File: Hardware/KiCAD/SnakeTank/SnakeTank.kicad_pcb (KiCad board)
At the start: 4 copper layers, 80.5 x 36.6 mm, 51 parts, among them J1 Conn_01x12, J2 USB_C_Receptacle_USB2.0_16P, J3 RJ45, Q1 L8050QLT1G, Q2 L8050QLT1G, U1 LP2985-3.3, U2 ESP32-S3-WROOM-1-N8, U4 FT231XS

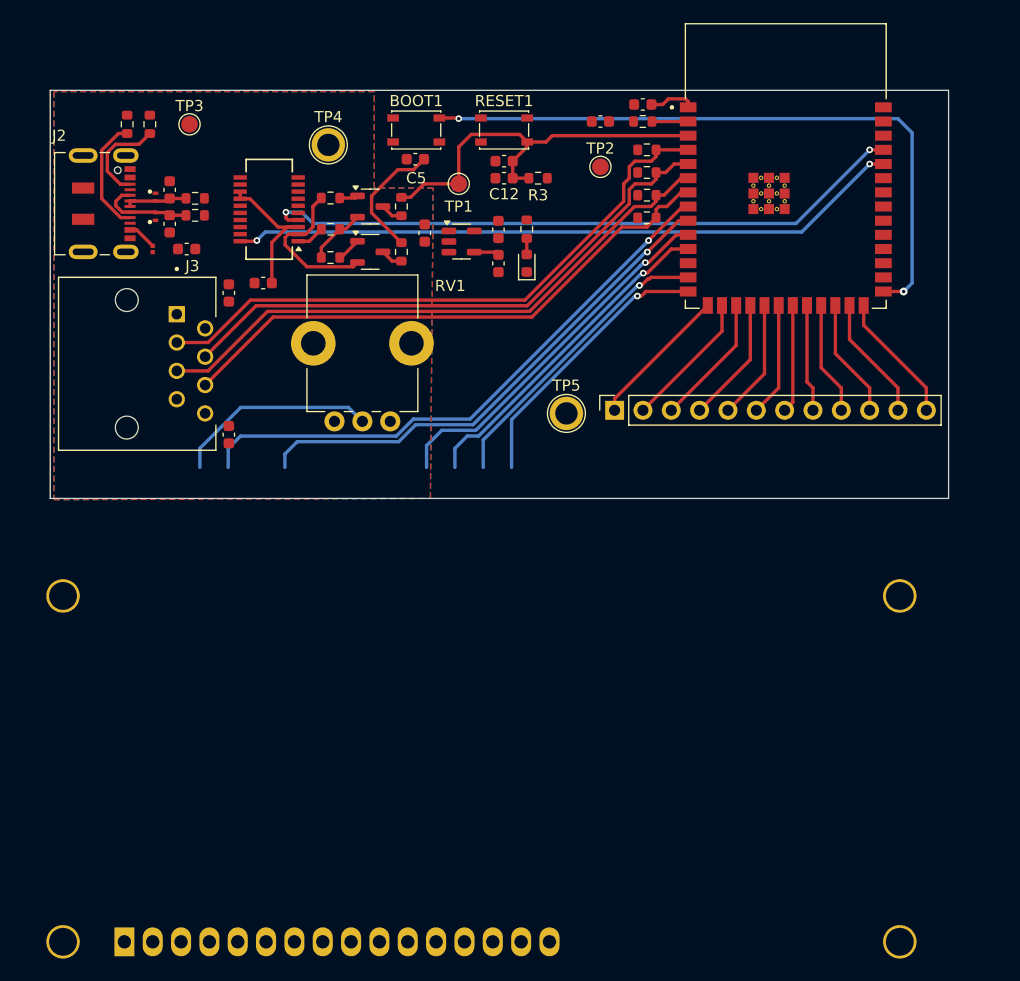
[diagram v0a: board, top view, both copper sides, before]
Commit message: WOOOHOO
rough draft of layout done
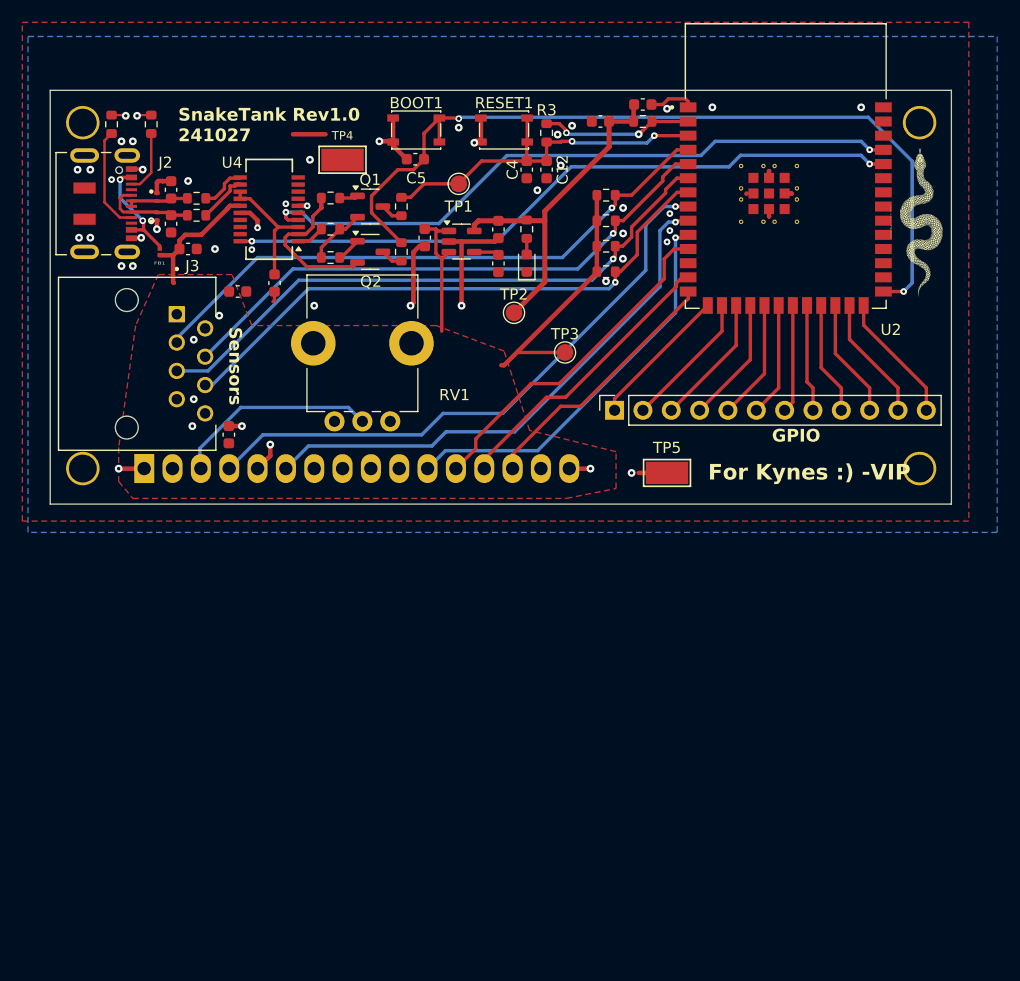
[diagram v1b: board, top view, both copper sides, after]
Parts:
- added G***: LOGO, graphics:snakeLogo, F.Cu at (95.9, 35.9)
- TP4, TP5: footprint TestPoint:TestPoint_Plated_Hole_D2.0mm -> TestPoint:TestPoint_Keystone_5019_Minature
- moved DS1 42.5 mm to (26.4, 58.0)
- moved TP3 39.4 mm to (64.1, 47.6)
- moved TP2 15.2 mm to (59.6, 44.1)
- moved TP5 10.5 mm to (73.3, 58.4)
- moved R12 6.05 mm to (67.8, 40.4)
- moved R13 5.85 mm to (67.8, 38.1)
- moved R14 5.66 mm to (67.8, 35.8)
- moved R15 5.47 mm to (67.8, 33.5)
- moved R3 4.13 mm to (62.5, 27.9), turned to -90 degrees
- moved C12 3.89 mm to (62.5, 31.2), turned to -90 degrees
- moved C4 2.17 mm to (60.7, 31.2), turned to -90 degrees
- moved TP4 1.84 mm to (44.2, 30.4)
- moved R1 1.40 mm to (23.5, 27.2)
- moved C7 1.02 mm to (38.1, 41.4), turned to -90 degrees
- moved C14 0.80 mm to (34.8, 42.2), turned to 0 degrees
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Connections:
- U2 pad 41_10: (no net) -> GND
- U2 pad 41_11: (no net) -> GND
- U2 pad 41_12: (no net) -> GND
- U2 pad 41_13: (no net) -> GND
- U2 pad 41_14: (no net) -> GND
- U2 pad 41_15: (no net) -> GND
- U2 pad 41_16: (no net) -> GND
- U2 pad 41_17: (no net) -> GND
- U2 pad 41_18: (no net) -> GND
- U2 pad 41_19: (no net) -> GND
- U2 pad 41_20: (no net) -> GND
- U2 pad 41_21: (no net) -> GND
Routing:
- net GND: track 4.21 -> 56.2 mm, vias 0 -> 51
- net +5V: track 0.00 -> 47.7 mm
- net +3.3V: track 0.00 -> 31.5 mm
- net ESP_3V3: track 3.60 -> 14.0 mm, vias 0 -> 2
- net Net-(FB1-Pad2): track 2.62 -> 9.85 mm, vias 0 -> 2
- net /GPIO_0: track 70.6 -> 75.7 mm
- net /USBN: track 0.00 -> 4.54 mm
- net /USBP: track 0.00 -> 4.12 mm
- net Net-(J2-CC1): track 8.70 -> 5.72 mm
- net LCD_D4: track 33.2 -> 36.0 mm
- net /CHIP_PU: track 36.4 -> 33.7 mm, vias 0 -> 2
- net LCD_E: track 46.0 -> 48.2 mm
- net Net-(U4-3V3OUT): track 13.5 -> 11.3 mm
- net LCD_RS: track 51.9 -> 53.2 mm
- net DHT11_4_data: track 50.9 -> 52.2 mm, vias 0 -> 1
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- added copper zone on B.Cu, net GND
- added copper zone on F.Cu, net GND
- added copper zone on In1.Cu, net GND
- added copper zone on In2.Cu, net GND
- removed copper zone on B.Cu, net +5V
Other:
- board size 80.5 x 36.6 mm -> 80.8 x 37.1 mm
- board text added: "For Kynes :) -VIP"
- board text added: "GPIO"
- board text added: "Sensors"
- board text added: "SnakeTank Rev1.0 241027"
